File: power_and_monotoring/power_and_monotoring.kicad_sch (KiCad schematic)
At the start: 4 parts

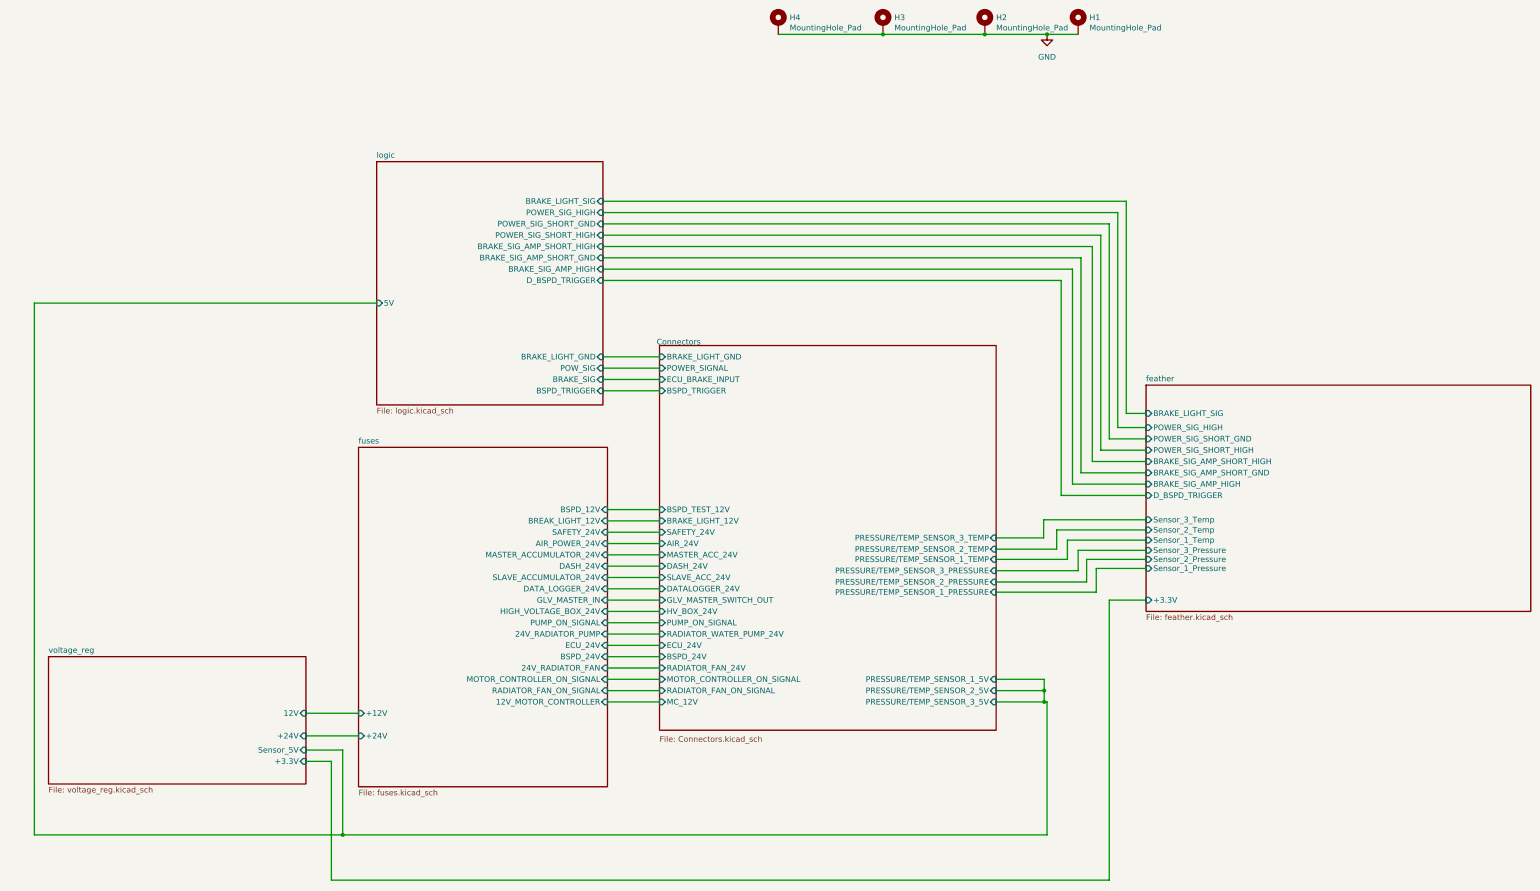
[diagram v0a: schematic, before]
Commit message: Final
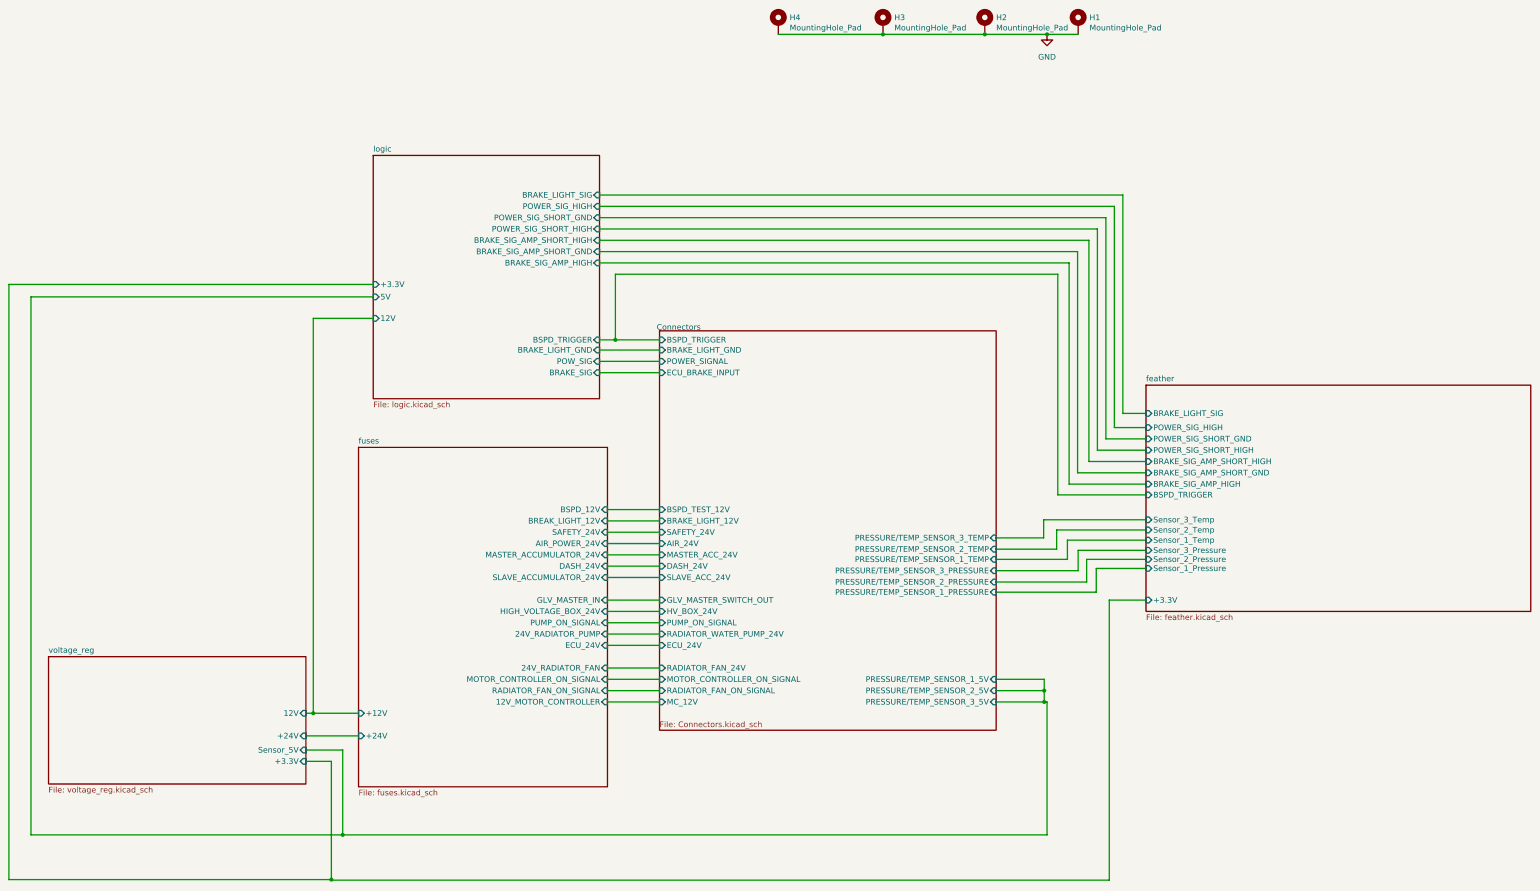
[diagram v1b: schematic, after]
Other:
- sheet Connectors ports: added none; removed BSPD_24V, DATALOGGER_24V
- sheet feather ports: added BSPD_TRIGGER; removed D_BSPD_TRIGGER
- sheet fuses ports: added none; removed BSPD_24V, DATA_LOGGER_24V
- sheet logic ports: added +3.3V, 12V; removed D_BSPD_TRIGGER
